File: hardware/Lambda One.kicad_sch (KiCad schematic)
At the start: 7 parts, among them IC1 01, J1 Conn_01x02, SW1 SW_Push, U1 W65C816SxP, U3 ATF22V10C, Y1 TFT680

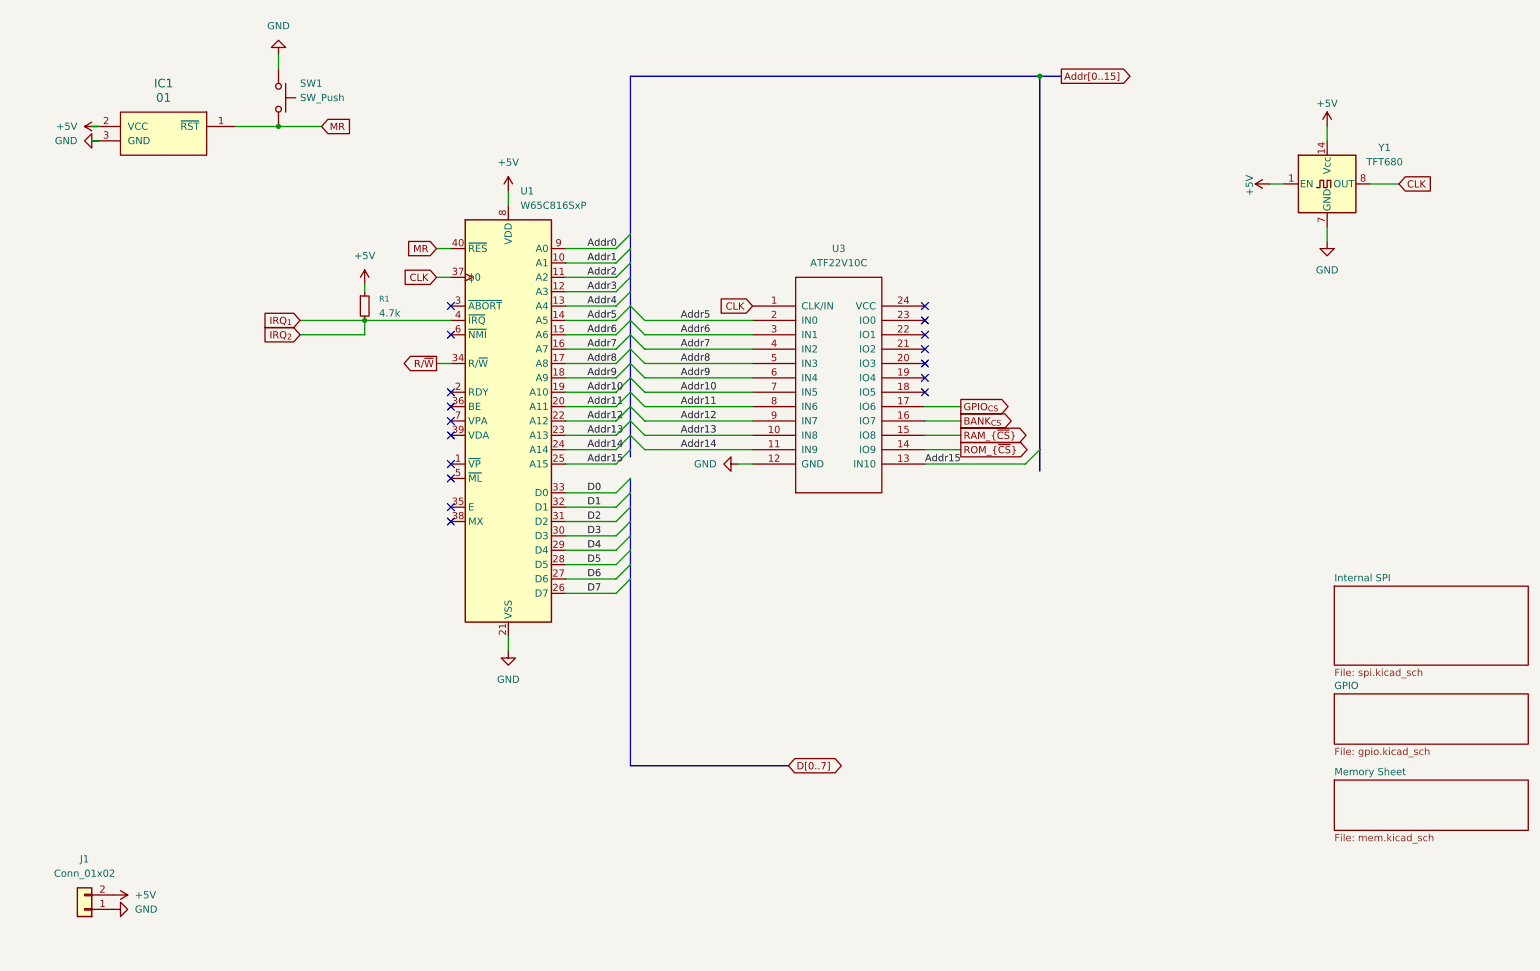
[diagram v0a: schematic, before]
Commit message: Added Board Register
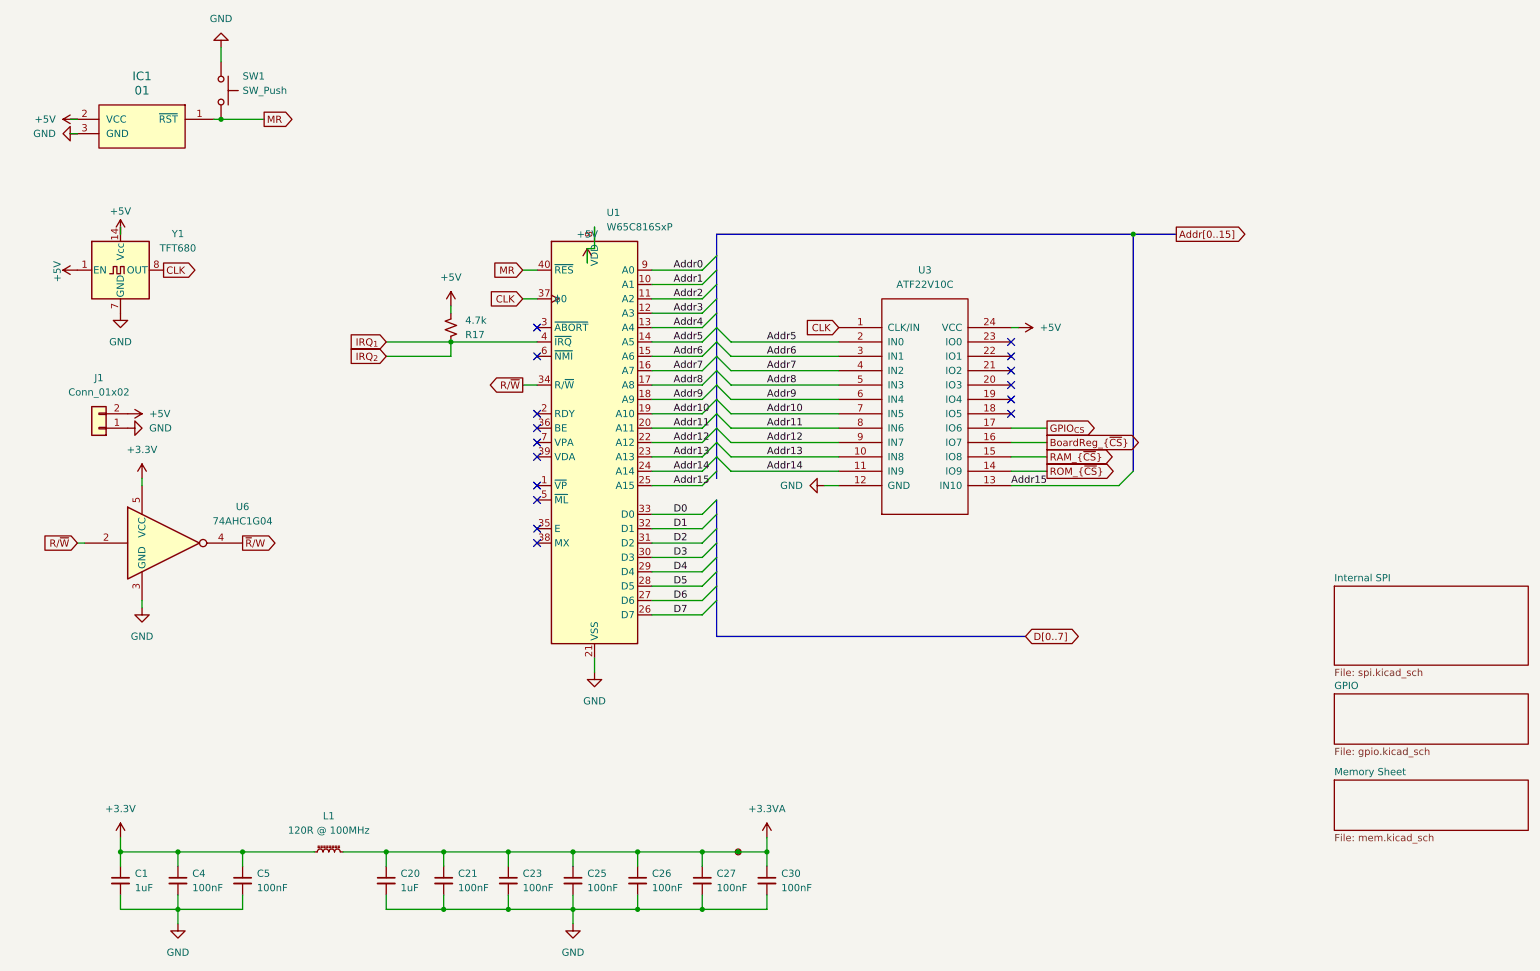
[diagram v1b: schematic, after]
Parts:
- removed R1: 4.7k, symbol Device:R_Small
- added C1, C20: 1uF, Capacitor_SMD:C_0603_1608Metric, symbol Device:C_Small
- added C21, C23, C25, C26, C27, C30, C4, C5: 100nF, Capacitor_SMD:C_0603_1608Metric, symbol Device:C_Small
- added L1: 120R @ 100MHz, Inductor_SMD:L_0603_1608Metric, symbol Device:L_Ferrite_Small
- added R17: 4.7k, Resistor_SMD:R_0603_1608Metric, symbol Device:R_Small_US
- added TP13: TestPoint_Small, TestPoint:TestPoint_Pad_D1.5mm, symbol Connector:TestPoint_Small
- added U6: 74AHC1G04, Package_TO_SOT_SMD:SOT-23-5, symbol 74xGxx:74AHC1G04
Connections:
- net +5V: now also U3.24 (VCC), R17.2
- net GND: now also C1.2, C20.2, C21.2, C23.2, C25.2, C26.2, C27.2, C30.2, C4.2, C5.2, U6.3 (GND)
- net IRQ_{1}: now also R17.1
- net R/~{W}: now also U6.2
- net BANK_{CS} renamed BoardReg_{~{CS}}
- new net +3.3V: C1.1, C4.1, C5.1, L1.1, U6.5 (VCC)
- new net +3.3VA: C20.1, C21.1, C23.1, C25.1, C26.1, C27.1, C30.1, L1.2, TP13.1
- new net ~{R}/W: U6.4
- no-connect marks 17 -> 16
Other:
- moved on the sheet: IC1, J1, SW1, U1, U3, Y1
